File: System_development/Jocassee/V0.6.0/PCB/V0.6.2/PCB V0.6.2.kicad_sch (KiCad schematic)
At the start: 8 parts, among them P1 ST-TF-003A, U1 NRF24L01_Breakout, U2 ProMicro, U3 EZO_PH, U4 EZO_TDS, U5 YAAJ_DCDC_StepDown_LM2596, U6 HX-2S-JH20

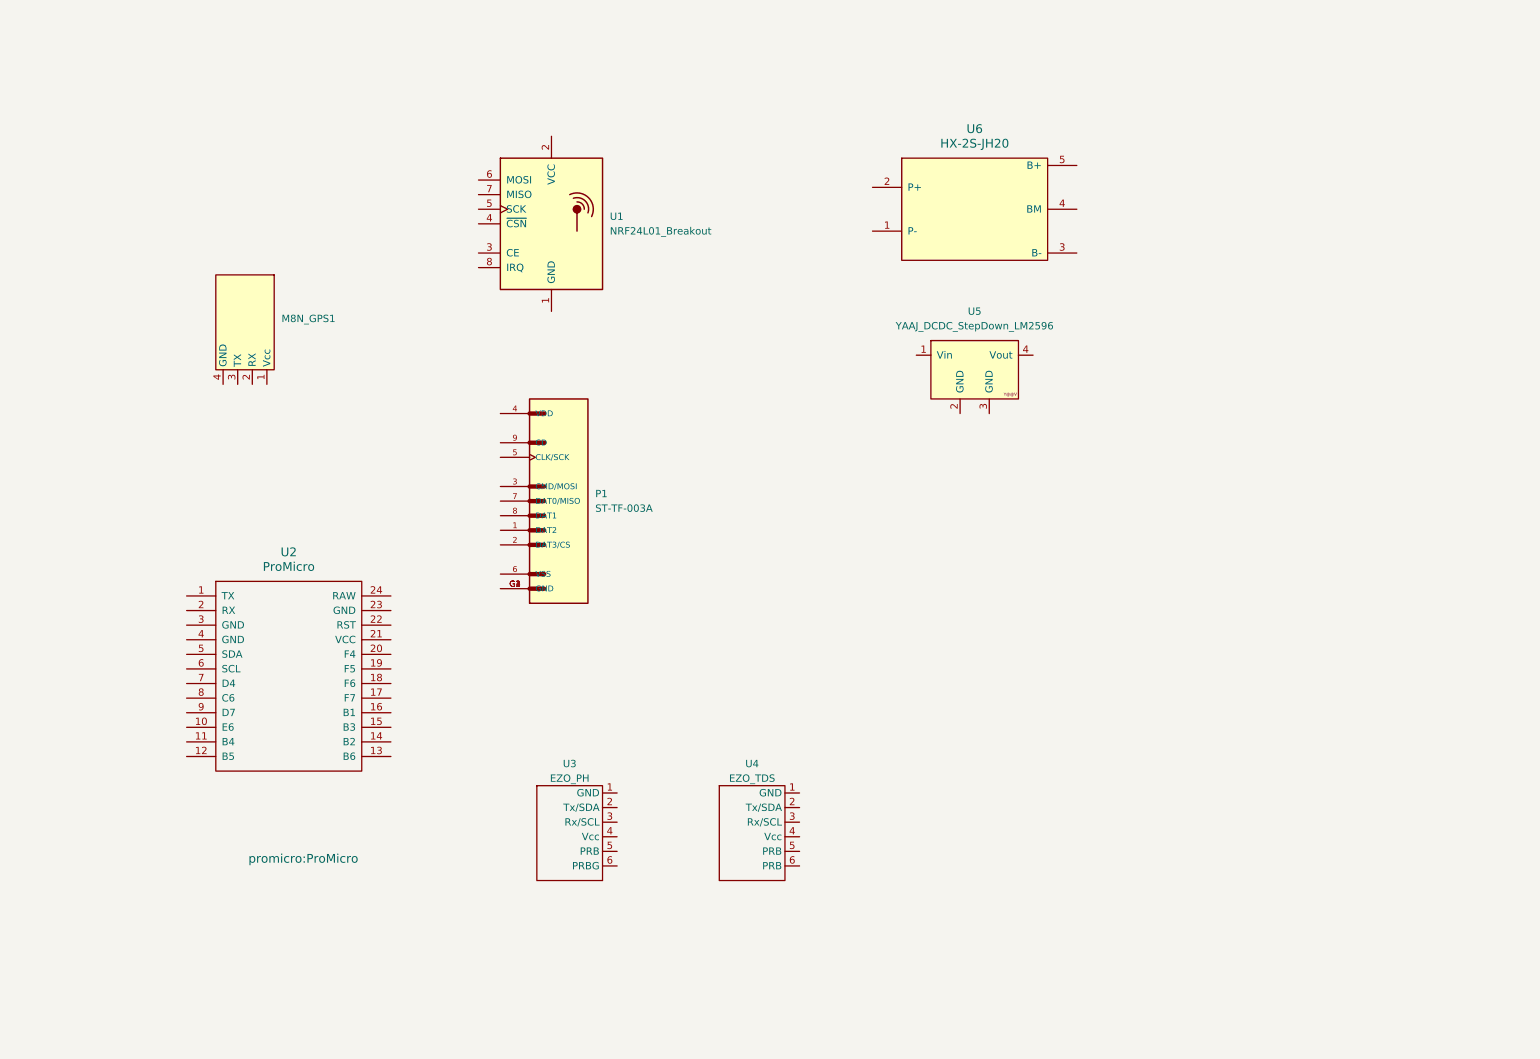
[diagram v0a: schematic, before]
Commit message: PCB routing done
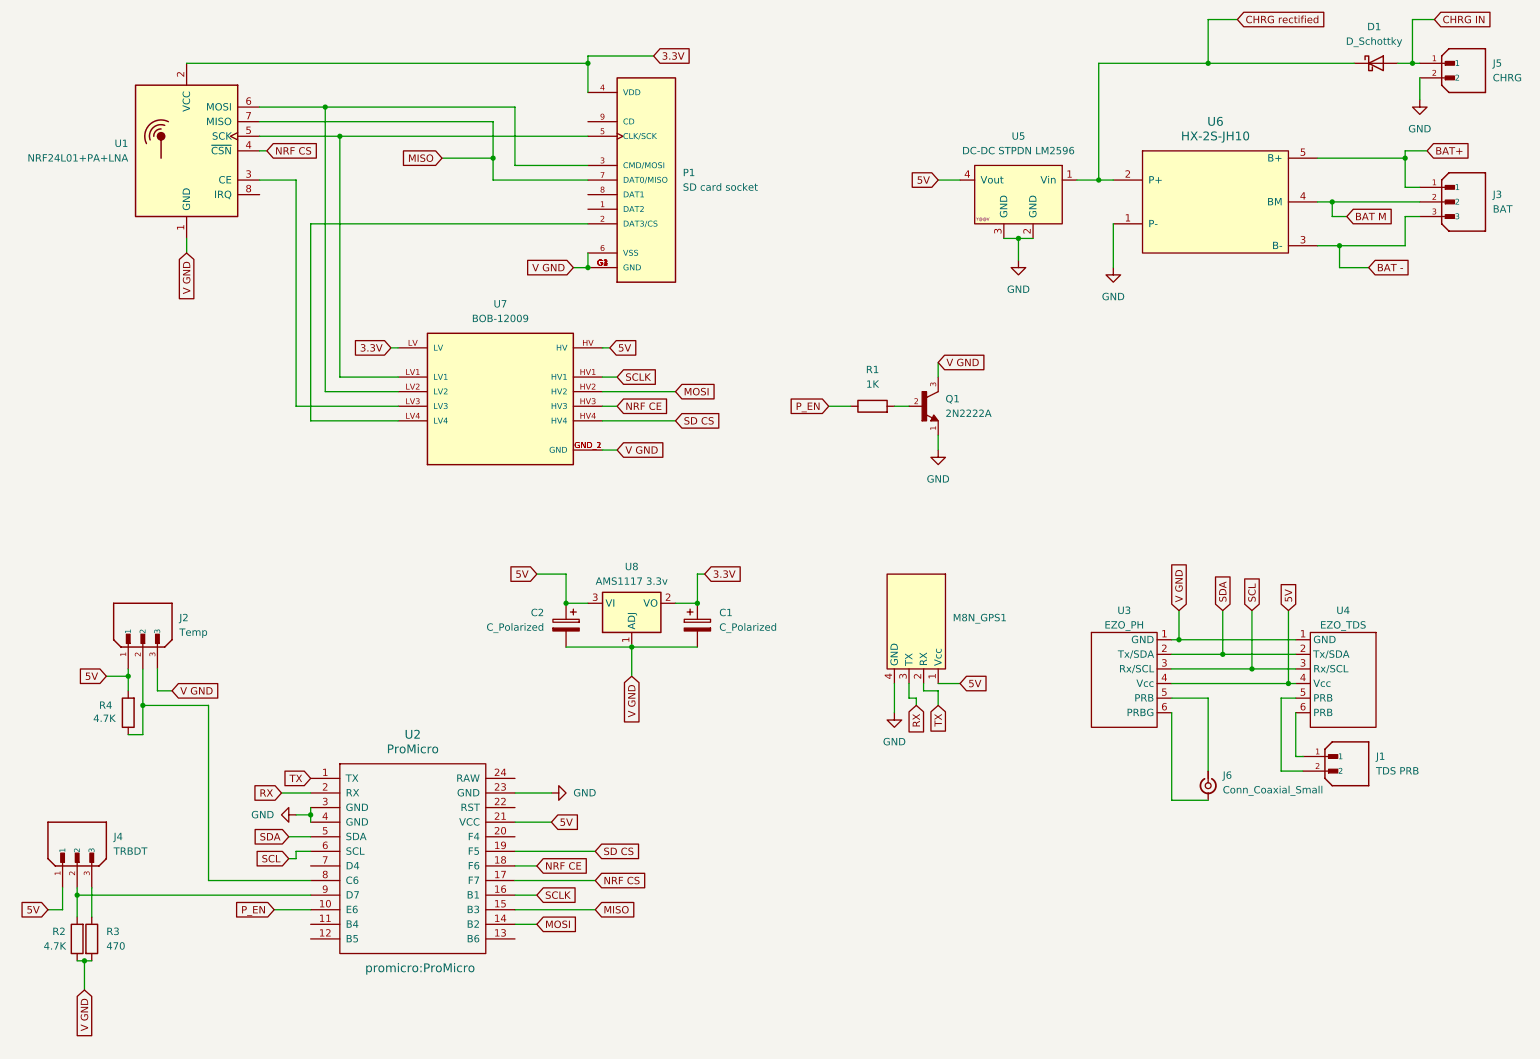
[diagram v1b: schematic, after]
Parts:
- removed U6: HX-2S-JH20, megasaturnv_custom_components:HX-2S-JH20, symbol megasaturnv_custom_components:HX-2S-JH20
- added C1, C2: C_Polarized, Capacitor_THT:CP_Radial_D4.0mm_P2.00mm, symbol Device:C_Polarized
- added D1: D_Schottky, Diode_THT:D_DO-34_SOD68_P7.62mm_Horizontal, symbol Device:D_Schottky
- added J1: TDS PRB, XH2.54 - 3pin:JST_B2B-XH-A_LF__SN_, symbol B2B-XH-A_LF__SN_:B2B-XH-A_LF__SN_
- added J2: Temp, XH2.54:XH2.54, symbol XH2.54:B3B-XH-A_LF__SN_
- added J3: BAT, XH2.54:XH2.54, symbol XH2.54:B3B-XH-A_LF__SN_
- added J4: TRBDT, XH2.54:XH2.54, symbol XH2.54:B3B-XH-A_LF__SN_
- added J5: CHRG, XH2.54 - 3pin:JST_B2B-XH-A_LF__SN_, symbol B2B-XH-A_LF__SN_:B2B-XH-A_LF__SN_
- added J6: Conn_Coaxial_Small, Connector_Coaxial:SMA_Amphenol_901-143_Horizontal, symbol Connector:Conn_Coaxial_Small
- added Q1: 2N2222A, 2N2222A:TO92254P470H750-3, symbol 2N2222A:2N2222A
- added R1: 1K, Resistor_THT:R_Axial_DIN0204_L3.6mm_D1.6mm_P5.08mm_Horizontal, symbol Device:R
- added R2: 4.7K, Resistor_THT:R_Axial_DIN0204_L3.6mm_D1.6mm_P7.62mm_Horizontal, symbol Device:R
- added R3: 470, Resistor_THT:R_Axial_DIN0204_L3.6mm_D1.6mm_P7.62mm_Horizontal, symbol Device:R
- added R4: 4.7K, Resistor_THT:R_Axial_DIN0204_L3.6mm_D1.6mm_P5.08mm_Horizontal, symbol Device:R
- added U6: HX-2S-JH10, megasaturnv_custom_components:HX-2S-JH10, symbol megasaturnv_custom_components:HX-2S-JH10
- added U7: BOB-12009, Logic level shifter:Logic_level_shifter, symbol Logic_level_shifter:BOB-12009
- added U8: AMS1117 3.3v, Package_TO_SOT_SMD:SOT-223-3_TabPin2, symbol Regulator_Linear:AMS1117
- P1: value ST-TF-003A -> SD card socket
- U1: value NRF24L01_Breakout -> NRF24L01+PA+LNA
- U5: value YAAJ_DCDC_StepDown_LM2596 -> DC-DC STPDN LM2596
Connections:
- net TX: now reaches U2.1 (TX)
- net TX: now also M8N_GPS1.2 (RX)
- net P_EN: now reaches U2.10 (E6)
- net P_EN: now also R1.1
- net MOSI: now reaches U2.14 (B2)
- net MOSI: now also U7.HV2
- net MISO: now reaches U2.15 (B3)
- net MISO: now also P1.7 (DAT0/MISO), U1.7 (MISO)
- net SCLK: now reaches U2.16 (B1)
- net SCLK: now also U7.HV1
- net NRF CS: now reaches U2.17 (F7)
- net NRF CS: now also U1.4 (~{CSN})
- net NRF CE: now reaches U2.18 (F6)
- net NRF CE: now also U7.HV3
- net SD CS: now reaches U2.19 (F5)
- net SD CS: now also U7.HV4
- net RX: now reaches U2.2 (RX)
- net RX: now also M8N_GPS1.3 (TX)
- net 5V: now reaches U2.21 (VCC)
- net 5V: now also M8N_GPS1.1 (Vcc), U3.4 (Vcc), U4.4 (Vcc), U5.4 (Vout), C2.1, J2.1, J4.1, R4.2, U7.HV, U8.3 (VI)
- net GND: now reaches U2.23 (GND)
- net GND: now also M8N_GPS1.4 (GND), U2.3 (GND), U2.4 (GND), U5.2 (GND), U5.3 (GND), J5.2, Q1.1, U6.1 (P-)
- net SDA: now reaches U2.5 (SDA)
- net SDA: now also U3.2 (Tx/SDA), U4.2 (Tx/SDA)
- net SCL: now reaches U2.6 (SCL)
- net SCL: now also U3.3 (Rx/SCL), U4.3 (Rx/SCL)
- net at U2.8 (C6): now also J2.2, R4.1
- net at U2.9 (D7): now also J4.2, R2.2
- net V GND: now reaches U3.1 (GND)
- net V GND: now also P1.6 (VSS), P1.G1 (GND), P1.G2 (GND), P1.G3 (GND), P1.G4 (GND), U1.1 (GND), U4.1 (GND), C1.2, C2.2, J2.3, Q1.3, R2.1, R3.2, U7.GND_1 (GND), U7.GND_2 (GND), U8.1 (ADJ)
- net at U3.5 (PRB): now also J6.1 (In)
- net at U3.6 (PRBG): now also J6.2 (Ext)
- net 3.3V: now reaches U1.2 (VCC)
- net 3.3V: now also P1.4 (VDD), C1.1, U7.LV, U8.2 (VO)
- net at U1.3 (CE): now also U7.LV3
- net at U1.5 (SCK): now also P1.5 (CLK/SCK), U7.LV1
- net at U1.6 (MOSI): now also P1.3 (CMD/MOSI), U7.LV2
- net at U4.5 (PRB): now also J1.2
- net at U4.6 (PRB): now also J1.1
- net at P1.2 (DAT3/CS): now also U7.LV4
- net CHRG rectified: now reaches U5.1 (Vin)
- net CHRG rectified: now also D1.1 (K), U6.2 (P+)
- new net: Q1.2, R1.2
- new net: J4.3, R3.1
- new net BAT -: J3.3, U6.3 (B-)
- new net BAT M: J3.2, U6.4 (BM)
- new net BAT+: J3.1, U6.5 (B+)
- new net CHRG IN: D1.2 (A), J5.1
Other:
- moved on the sheet: M8N_GPS1, U1, U2, U3, U4, U5
